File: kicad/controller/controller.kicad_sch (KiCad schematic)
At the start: 10 parts, among them J1 Conn_01x07_Male, U1 BluePill_STM32F103C

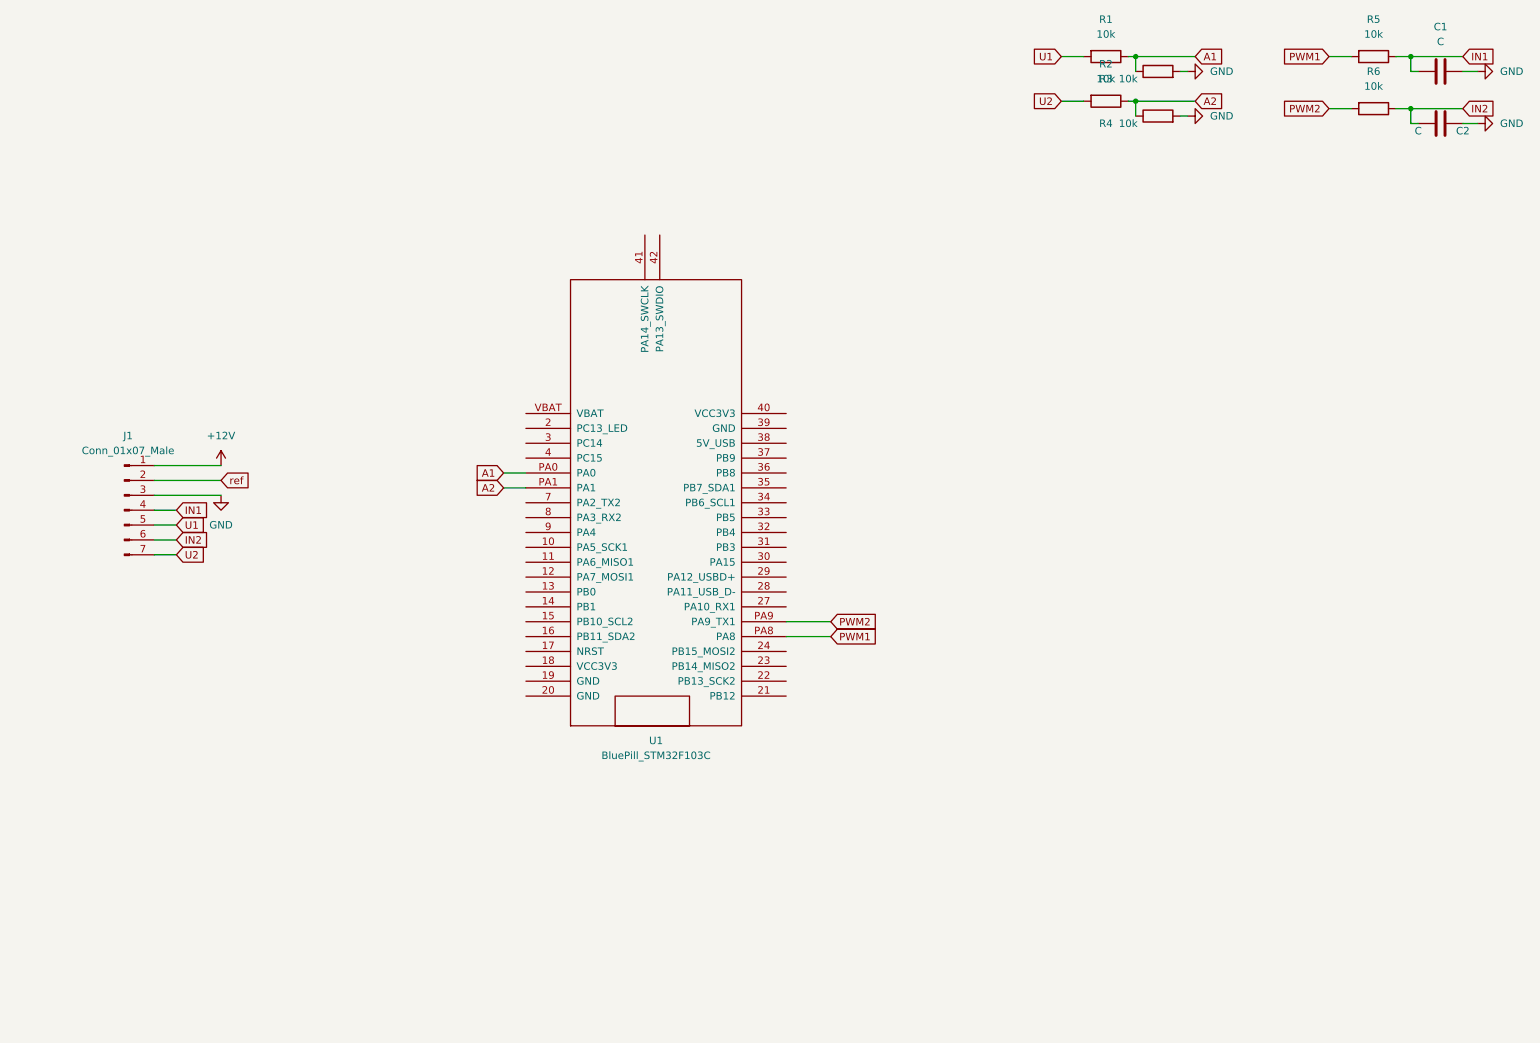
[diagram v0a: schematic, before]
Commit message: work on kicad
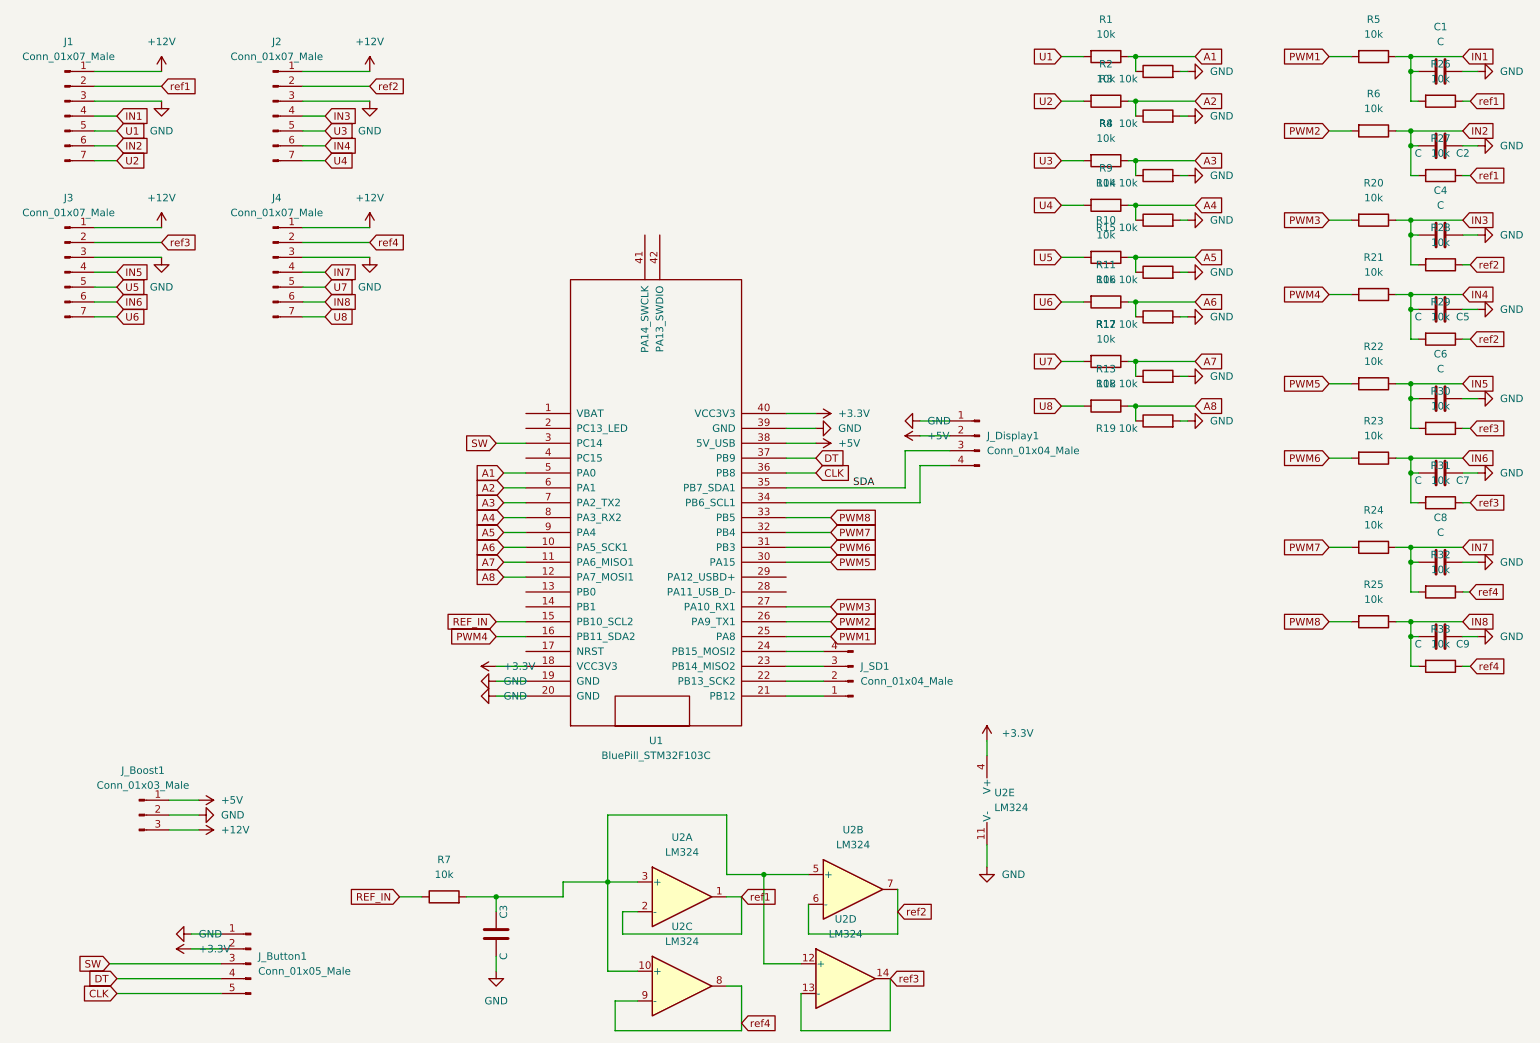
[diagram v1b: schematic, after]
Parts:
- added C3, C4, C5, C6, C7, C8, C9: C, Capacitor_SMD:C_0805_2012Metric, symbol Device:C
- added J2, J3, J4: Conn_01x07_Male, Connector_PinHeader_2.54mm:PinHeader_1x07_P2.54mm_Vertical, symbol Connector:Conn_01x07_Male
- added J_Boost1: Conn_01x03_Male, Connector_PinHeader_2.54mm:PinHeader_1x03_P2.54mm_Vertical, symbol Connector:Conn_01x03_Male
- added J_Button1: Conn_01x05_Male, Connector_PinHeader_2.54mm:PinHeader_1x05_P2.54mm_Vertical, symbol Connector:Conn_01x05_Male
- added J_Display1, J_SD1: Conn_01x04_Male, Connector_PinHeader_2.54mm:PinHeader_1x04_P2.54mm_Vertical, symbol Connector:Conn_01x04_Male
- added R10, R11, R12, R13, R14, R15, R16, R17, R18, R19, R20, R21, R22, R23, R24, R25, R26, R27, R28, R29, R30, R31, R32, R33, R7, R8, R9: 10k, Resistor_SMD:R_1206_3216Metric, symbol Device:R
- added U2: LM324, Package_SO:SOIC-14_3.9x8.7mm_P1.27mm, symbol Amplifier_Operational:LM324
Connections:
- net +12V: now also J2.1 (Pin_1), J3.1 (Pin_1), J4.1 (Pin_1), J_Boost1.3 (Pin_3)
- net A1: now also U1.5 (PA0); no longer U1.PA0
- net A2: now also U1.6 (PA1); no longer U1.PA1
- net GND: now also U1.19 (GND), U1.20 (GND), U1.39 (GND), C3.1, C4.2, C5.2, C6.2, C7.2, C8.2, C9.2, J2.3 (Pin_3), J3.3 (Pin_3), J4.3 (Pin_3), J_Boost1.2 (Pin_2), J_Button1.1 (Pin_1), J_Display1.1 (Pin_1), R14.2, R15.2, R16.2, R17.2, R18.2, R19.2, U2.11 (V-)
- net IN1: now also R26.2
- net IN2: now also R27.2
- net PWM1: now also U1.25 (PA8); no longer U1.PA8
- net PWM2: now also U1.26 (PA9_TX1); no longer U1.PA9 (PA9_TX1)
- net A6: now reaches U1.10 (PA5_SCK1)
- net A6: now also R11.1, R17.1
- net A7: now reaches U1.11 (PA6_MISO1)
- net A7: now also R12.1, R18.1
- net A8: now reaches U1.12 (PA7_MOSI1)
- net A8: now also R13.1, R19.1
- net REF_IN: now reaches U1.15 (PB10_SCL2)
- net REF_IN: now also R7.1
- net PWM4: now reaches U1.16 (PB11_SDA2)
- net PWM4: now also R21.2
- net +3.3V: now reaches U1.18 (VCC3V3)
- net +3.3V: now also U1.40 (VCC3V3), J_Button1.2 (Pin_2), U2.4 (V+)
- net at U1.21 (PB12): now also J_SD1.1 (Pin_1)
- net at U1.22 (PB13_SCK2): now also J_SD1.2 (Pin_2)
- net at U1.23 (PB14_MISO2): now also J_SD1.3 (Pin_3)
- net at U1.24 (PB15_MOSI2): now also J_SD1.4 (Pin_4)
- net PWM3: now reaches U1.27 (PA10_RX1)
- net PWM3: now also R20.2
- net SW: now reaches U1.3 (PC14)
- net SW: now also J_Button1.3 (Pin_3)
- net PWM5: now reaches U1.30 (PA15)
- net PWM5: now also R22.2
- net PWM6: now reaches U1.31 (PB3)
- net PWM6: now also R23.2
- net PWM7: now reaches U1.32 (PB4)
- net PWM7: now also R24.2
- net PWM8: now reaches U1.33 (PB5)
- net PWM8: now also R25.2
- net at U1.34 (PB6_SCL1): now also J_Display1.4 (Pin_4)
- net SDA: now reaches U1.35 (PB7_SDA1)
- net SDA: now also J_Display1.3 (Pin_3)
- net CLK: now reaches U1.36 (PB8)
- net CLK: now also J_Button1.5 (Pin_5)
- net DT: now reaches U1.37 (PB9)
- net DT: now also J_Button1.4 (Pin_4)
- net +5V: now reaches U1.38 (5V_USB)
- net +5V: now also J_Boost1.1 (Pin_1), J_Display1.2 (Pin_2)
- net A3: now reaches U1.7 (PA2_TX2)
- net A3: now also R14.1, R8.1
- net A4: now reaches U1.8 (PA3_RX2)
- net A4: now also R15.1, R9.1
- net A5: now reaches U1.9 (PA4)
- net A5: now also R10.1, R16.1
- net ref renamed ref1
- net ref1: now also R26.1, R27.1, U2.1, U2.2 (-)
- new net: C3.2, R7.2, U2.10 (+), U2.12 (+), U2.3 (+), U2.5 (+)
- new net IN3: C4.1, J2.4 (Pin_4), R20.1, R28.2
- new net IN4: C5.1, J2.6 (Pin_6), R21.1, R29.2
- new net IN5: C6.1, J3.4 (Pin_4), R22.1, R30.2
- new net IN6: C7.1, J3.6 (Pin_6), R23.1, R31.2
- new net IN7: C8.1, J4.4 (Pin_4), R24.1, R32.2
- new net IN8: C9.1, J4.6 (Pin_6), R25.1, R33.2
- new net U3: J2.5 (Pin_5), R8.2
- new net U4: J2.7 (Pin_7), R9.2
- new net U5: J3.5 (Pin_5), R10.2
- new net U6: J3.7 (Pin_7), R11.2
- new net U7: J4.5 (Pin_5), R12.2
- new net U8: J4.7 (Pin_7), R13.2
- new net ref2: J2.2 (Pin_2), R28.1, R29.1, U2.6 (-), U2.7
- new net ref3: J3.2 (Pin_2), R30.1, R31.1, U2.13 (-), U2.14
- new net ref4: J4.2 (Pin_2), R32.1, R33.1, U2.8, U2.9 (-)
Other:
- moved on the sheet: C2, J1, R6
